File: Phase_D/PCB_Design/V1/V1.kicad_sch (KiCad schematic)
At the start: 2 parts

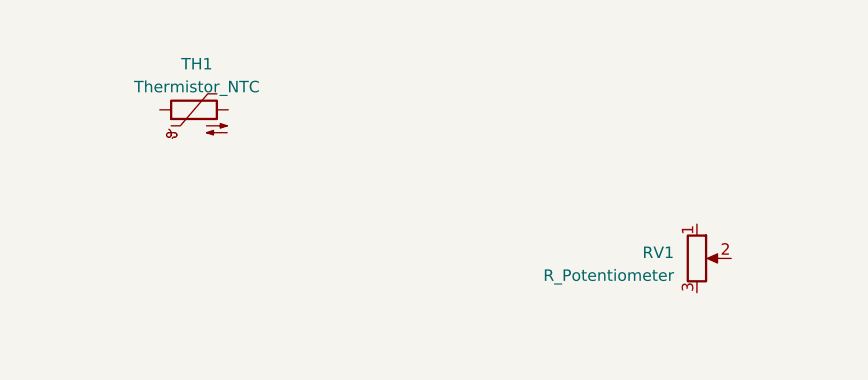
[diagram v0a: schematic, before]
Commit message: Prototype Update
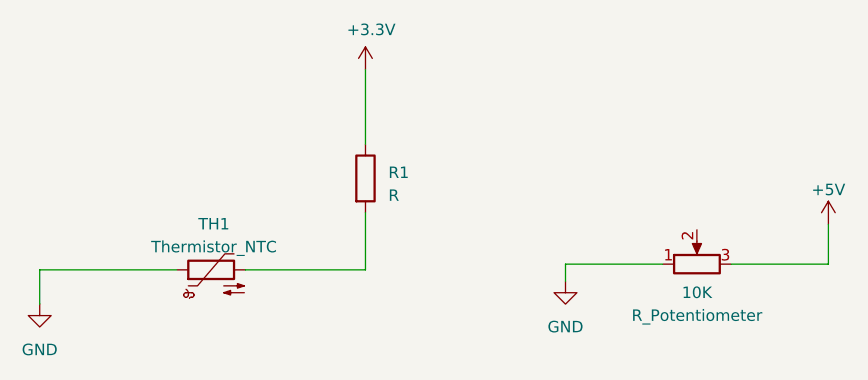
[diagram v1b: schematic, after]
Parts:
- added R1: R, symbol Device:R
- renumbered RV1 to 10K
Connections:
- net GND: now reaches TH1.1
- net GND: now also 10K.1
- net at TH1.2: now also R1.2
- net +5V: now reaches 10K.3
- new net +3.3V: R1.1
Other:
- moved on the sheet: 10K, TH1
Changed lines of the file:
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@@
 (kicad_sch (version 20230121) (generator eeschema)
   (paper "A4")
-  (symbol (lib_id "Device:Thermistor_NTC") (at 88.9 74.93 90) (unit 1)
+  (wire (pts (xy 107.95 92.71) (xy 94.615 92.71))
+    (stroke (width 0) (type default))
+  )
+  (wire (pts (xy 107.95 70.485) (xy 107.95 78.74))
+    (stroke (width 0) (type default))
+  )
+  (wire (pts (xy 159.385 92.075) (xy 159.385 87.63))
+    (stroke (width 0) (type default))
+  )
+  (wire (pts (xy 71.755 92.71) (xy 71.755 96.52))
+    (stroke (width 0) (type default))
+  )
+  (wire (pts (xy 148.59 92.075) (xy 159.385 92.075))
+    (stroke (width 0) (type default))
+  )
+  (wire (pts (xy 86.995 92.71) (xy 71.755 92.71))
+    (stroke (width 0) (type default))
+  )
+  (wire (pts (xy 107.95 86.36) (xy 107.95 92.71))
+    (stroke (width 0) (type default))
+  )
+  (wire (pts (xy 130.175 92.075) (xy 130.175 93.98))
+    (stroke (width 0) (type default))
+  )
+  (wire (pts (xy 140.97 92.075) (xy 130.175 92.075))
+    (stroke (width 0) (type default))
+  )
+  (symbol (lib_id "Device:Thermistor_NTC") (at 90.805 92.71 90) (unit 1)
     (in_bom yes) (on_board yes) (dnp no) (fields_autoplaced)
-    (property "Reference" "TH1" (at 89.2175 69.85 90)
+    (property "Reference" "TH1" (at 91.1225 87.63 90)
       (effects (font (size 1.27 1.27)))
     )
-    (property "Value" "Thermistor_NTC" (at 89.2175 72.39 90)
+    (property "Value" "Thermistor_NTC" (at 91.1225 90.17 90)
       (effects (font (size 1.27 1.27)))
     )
-    (property "Footprint" "" (at 87.63 74.93 0)
+    (property "Footprint" "" (at 89.535 92.71 0)
       (effects (font (size 1.27 1.27)) hide)
     )
-    (property "Datasheet" "~" (at 87.63 74.93 0)
+    (property "Datasheet" "~" (at 89.535 92.71 0)
       (effects (font (size 1.27 1.27)) hide)
     )
@@
     )
   )
-  (symbol (lib_id "Device:R_Potentiometer") (at 144.78 91.44 0) (unit 1)
+  (symbol (lib_id "Device:R_Potentiometer") (at 144.78 92.075 90) (unit 1)
     (in_bom yes) (on_board yes) (dnp no) (fields_autoplaced)
-    (property "Reference" "RV1" (at 142.24 90.805 0)
-      (effects (font (size 1.27 1.27)) (justify right))
+    (property "Reference" "10K" (at 144.78 95.25 90)
+      (effects (font (size 1.27 1.27)))
     )
-    (property "Value" "R_Potentiometer" (at 142.24 93.345 0)
-      (effects (font (size 1.27 1.27)) (justify right))
+    (property "Value" "R_Potentiometer" (at 144.78 97.79 90)
+      (effects (font (size 1.27 1.27)))
     )
-    (property "Footprint" "" (at 144.78 91.44 0)
+    (property "Footprint" "" (at 144.78 92.075 0)
       (effects (font (size 1.27 1.27)) hide)
     )
-    (property "Datasheet" "~" (at 144.78 91.44 0)
+    (property "Datasheet" "~" (at 144.78 92.075 0)
       (effects (font (size 1.27 1.27)) hide)
     )
@@
       (project "V1"
         (path "/bf667db7-508f-459e-90e5-7585272ae06a"
-          (reference "RV1") (unit 1)
+          (reference "10K") (unit 1)
         )
       )
+    )
+  )
+  (symbol (lib_id "power:+5V") (at 159.385 87.63 0) (unit 1)
+    (in_bom yes) (on_board yes) (dnp no) (fields_autoplaced)
+    (property "Reference" "#PWR02" (at 159.385 91.44 0)
+      (effects (font (size 1.27 1.27)) hide)
+    )
+    (property "Value" "+5V" (at 159.385 83.82 0)
+      (effects (font (size 1.27 1.27)))
+    )
+    (property "Footprint" "" (at 159.385 87.63 0)
+      (effects (font (size 1.27 1.27)) hide)
+    )
+    (property "Datasheet" "" (at 159.385 87.63 0)
+      (effects (font (size 1.27 1.27)) hide)
+    )
+    (pin "1")
+    (instances
+      (project "V1"
+        (path "/bf667db7-508f-459e-90e5-7585272ae06a"
+          (reference "#PWR02") (unit 1)
+        )
+      )
+    )
+  )
+  (symbol (lib_id "Device:R") (at 107.95 82.55 0) (unit 1)
+    (in_bom yes) (on_board yes) (dnp no) (fields_autoplaced)
+    (property "Reference" "R1" (at 110.49 81.915 0)
+      (effects (font (size 1.27 1.27)) (justify left))
+    )
+    (property "Value" "R" (at 110.49 84.455 0)
+      (effects (font (size 1.27 1.27)) (justify left))
+    )
+    (property "Footprint" "" (at 106.172 82.55 90)
+      (effects (font (size 1.27 1.27)) hide)
+    )
+    (property "Datasheet" "~" (at 107.95 82.55 0)
+      (effects (font (size 1.27 1.27)) hide)
+    )
+    (pin "1")
+    (pin "2")
+    (instances
+      (project "V1"
+        (path "/bf667db7-508f-459e-90e5-7585272ae06a"
+          (reference "R1") (unit 1)
+        )
+      )
+    )
+  )
+  (symbol (lib_id "power:+3.3V") (at 107.95 70.485 0) (unit 1)
+    (in_bom yes) (on_board yes) (dnp no)
+    (property "Reference" "#PWR01" (at 107.95 74.295 0)
+      (effects (font (size 1.27 1.27)) hide)
+    )
+    (property "Value" "+3.3V" (at 108.585 66.04 0)
+      (effects (font (size 1.27 1.27)))
+    )
+    (property "Footprint" "" (at 107.95 70.485 0)
+      (effects (font (size 1.27 1.27)) hide)
+    )
+    (property "Datasheet" "" (at 107.95 70.485 0)
+      (effects (font (size 1.27 1.27)) hide)
+    )
+    (pin "1")
+    (instances
+      (project "V1"
+        (path "/bf667db7-508f-459e-90e5-7585272ae06a"
+          (reference "#PWR01") (unit 1)
+        )
+      )
+    )
+  )
+  (symbol (lib_id "power:GND") (at 130.175 93.98 0) (unit 1)
+    (in_bom yes) (on_board yes) (dnp no) (fields_autoplaced)
+    (property "Reference" "#PWR04" (at 130.175 100.33 0)
+      (effects (font (size 1.27 1.27)) hide)
+    )
+    (property "Value" "GND" (at 130.175 99.06 0)
+      (effects (font (size 1.27 1.27)))
+    )
+    (property "Footprint" "" (at 130.175 93.98 0)
+      (effects (font (size 1.27 1.27)) hide)
+    )
+    (property "Datasheet" "" (at 130.175 93.98 0)
+      (effects (font (size 1.27 1.27)) hide)
+    )
+    (pin "1")
+    (instances
+      (project "V1"
+        (path "/bf667db7-508f-459e-90e5-7585272ae06a"
+          (reference "#PWR04") (unit 1)
+        )
+      )
+    )
+  )
+  (symbol (lib_id "power:GND") (at 71.755 96.52 0) (unit 1)
+    (in_bom yes) (on_board yes) (dnp no) (fields_autoplaced)
+    (property "Reference" "#PWR03" (at 71.755 102.87 0)
+      (effects (font (size 1.27 1.27)) hide)
+    )
+    (property "Value" "GND" (at 71.755 101.6 0)
+      (effects (font (size 1.27 1.27)))
+    )
+    (property "Footprint" "" (at 71.755 96.52 0)
+      (effects (font (size 1.27 1.27)) hide)
+    )
+    (property "Datasheet" "" (at 71.755 96.52 0)
+      (effects (font (size 1.27 1.27)) hide)
+    )
+    (pin "1")
+    (instances
+      (project "V1"
+        (path "/bf667db7-508f-459e-90e5-7585272ae06a"
+          (reference "#PWR03") (unit 1)
+        )
+      )
